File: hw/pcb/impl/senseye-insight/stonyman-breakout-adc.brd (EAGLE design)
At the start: 30.5 x 9.8 mm, 8 parts

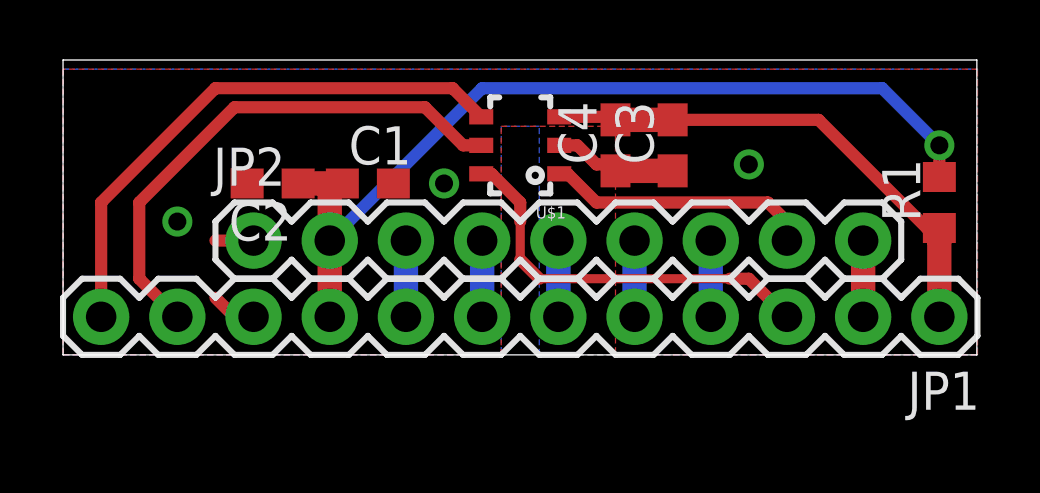
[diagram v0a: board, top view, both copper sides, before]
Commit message: added one more extra piece of GND routing
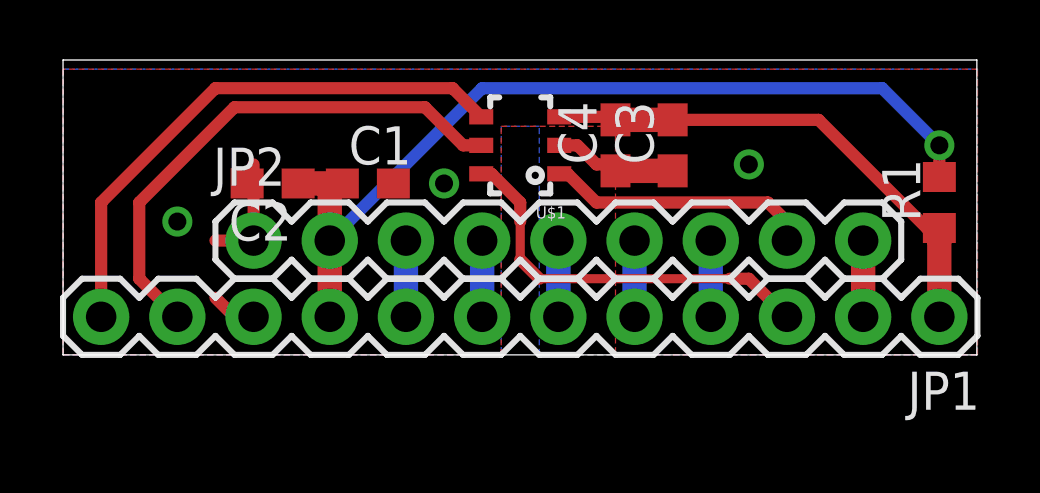
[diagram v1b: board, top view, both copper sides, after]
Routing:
- net GND: track 6.94 -> 9.48 mm
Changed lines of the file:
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@@
 <via x="12.7" y="5.715" extent="1-16" drill="0.6"/>
 <via x="3.81" y="4.445" extent="1-16" drill="0.6"/>
+<wire x1="6.35" y1="3.81" x2="6.35" y2="6.35" width="0.4064" layer="1"/>
 </signal>
 <signal name="V_STONY">
